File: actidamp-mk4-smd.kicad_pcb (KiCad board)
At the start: 2 copper layers, 119 x 100 mm, 199 parts, among them J101 XLR3, J102 Phono_Ground, J103 PHONO_IN_L, J104 PHONO_IN_R, J105 LINE_OUT_L, J106 LINE_OUT_R, Q201 2SK3320, Q301 2SK3320, Q401 BC846BPN, Q501 BC846BPN, SW201 SW_DIP_x04, SW202 SW_DPDT_x2, SW301 SW_DIP_x04, U101 LM317_3PinPackage, U102 LM337_TO252, U201 NE5532, U202 NE5534, U203 LF411, U204 NE5532, U205 LF411, U301 NE5532, U302 NE5534, U303 LF411, U304 NE5532, U305 LF411

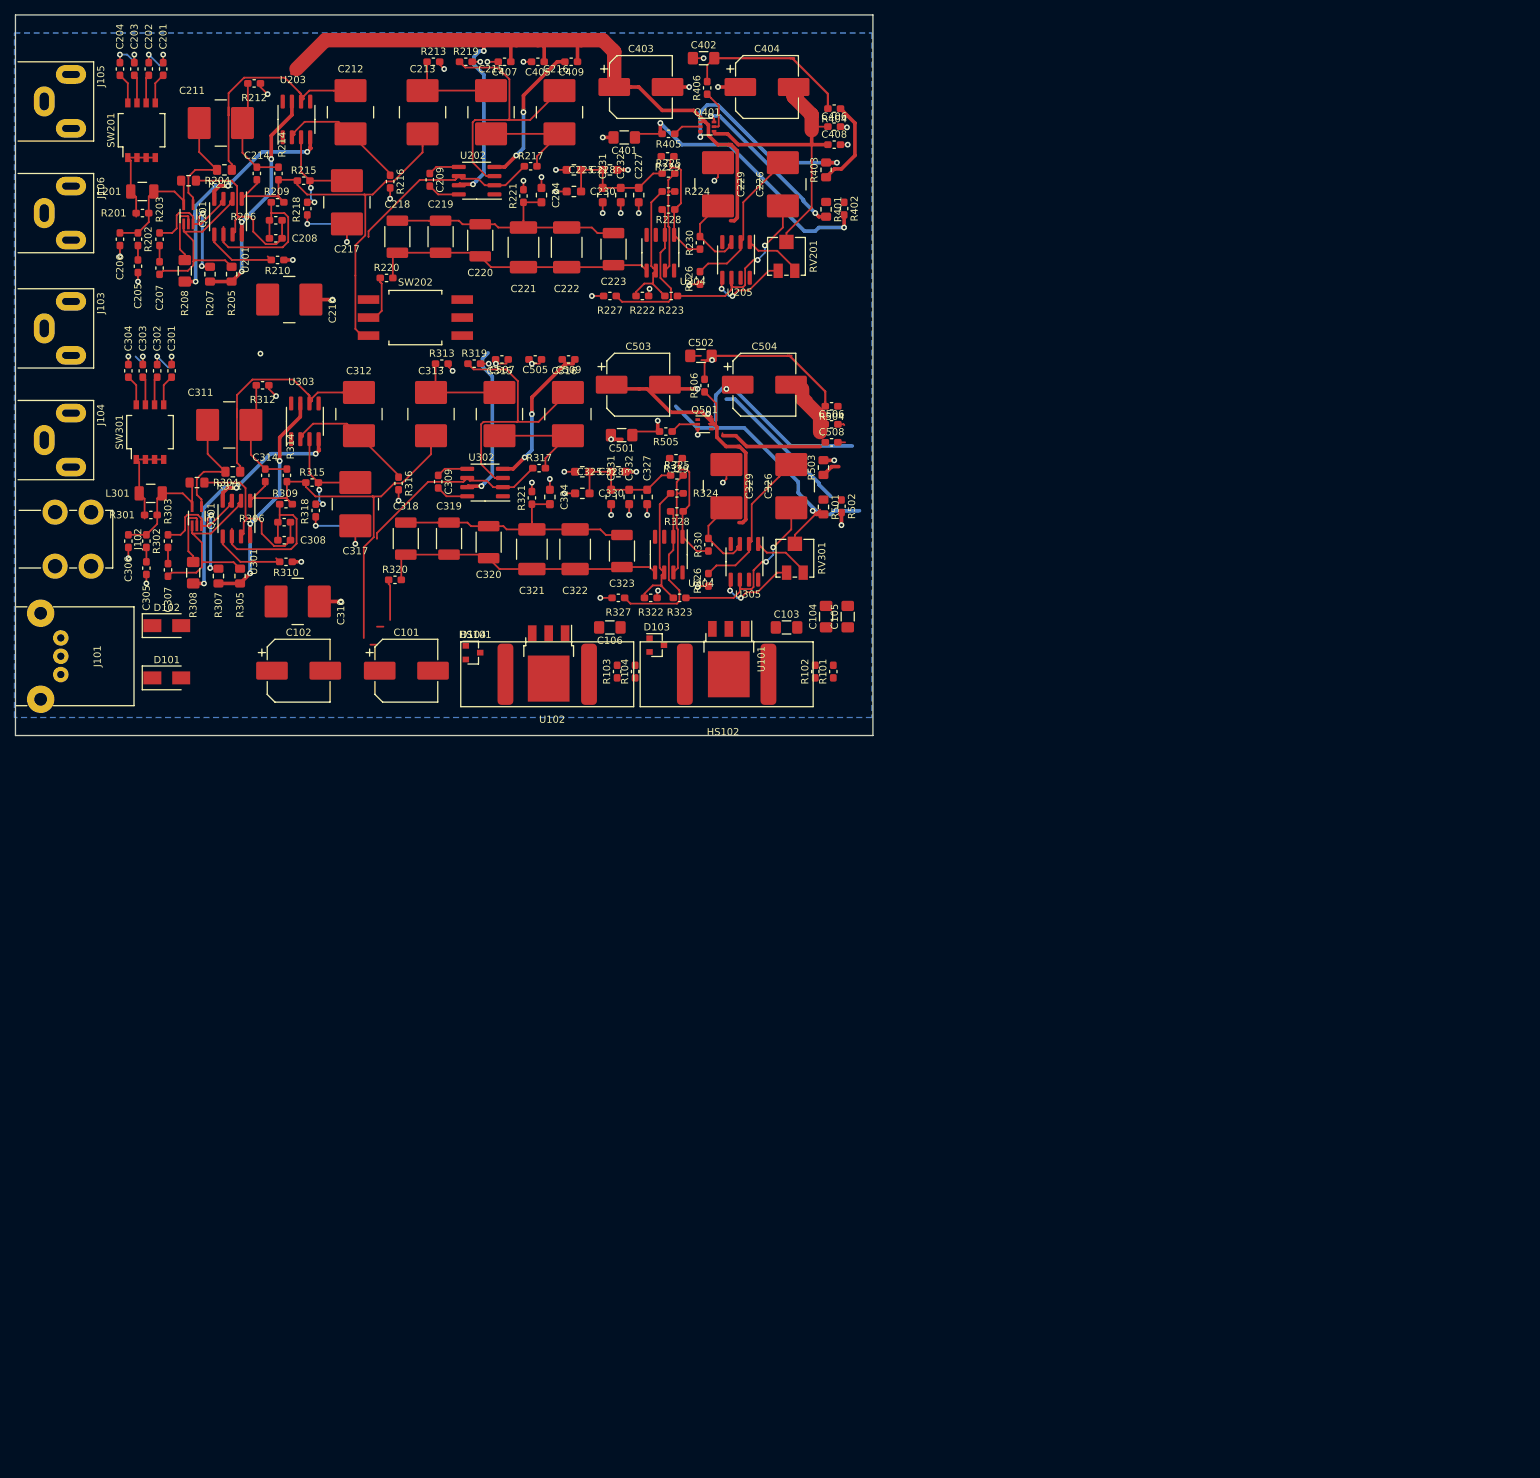
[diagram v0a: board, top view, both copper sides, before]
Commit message: All routed
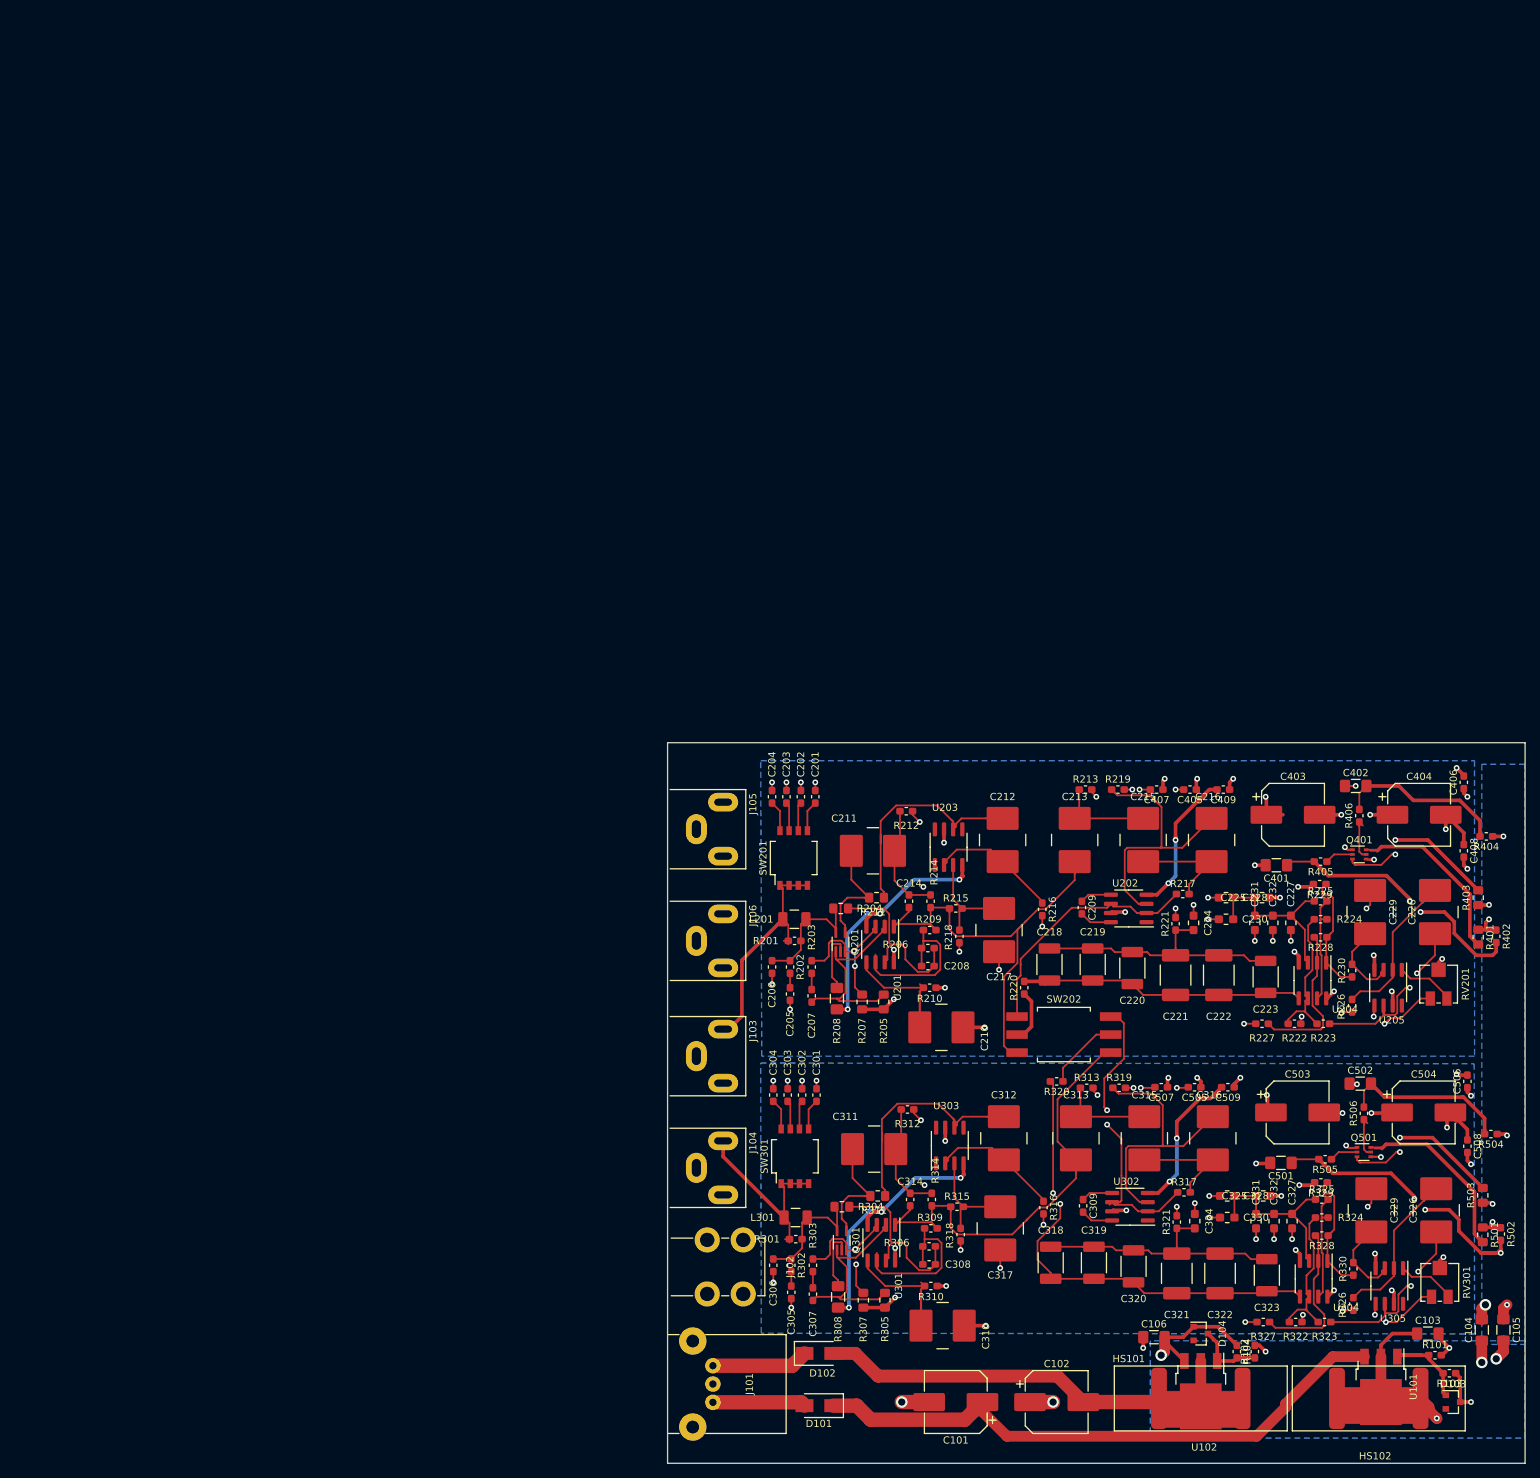
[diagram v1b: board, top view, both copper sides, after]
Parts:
- moved D103 152.5 mm to (199.5, 142.5)
- moved R103 151.1 mm to (199.0, 138.5), turned to 180 degrees
- moved C102 146.2 mm to (144.5, 142.5)
- moved D104 138.3 mm to (164.5, 133.0)
- moved C501 136.3 mm to (175.6, 109.3)
- moved C502 136.3 mm to (186.6, 98.3)
- moved C503 136.3 mm to (177.9, 102.3)
- moved C504 136.3 mm to (195.4, 102.3)
- moved C505 136.3 mm to (163.6, 98.8)
- moved C507 136.3 mm to (159.0, 98.8)
- moved C509 136.3 mm to (168.3, 98.8)
- moved Q501 136.3 mm to (187.1, 107.8)
- moved R501 136.3 mm to (203.6, 119.3)
- moved R502 136.3 mm to (206.1, 119.2)
- moved R503 136.3 mm to (203.6, 113.8)
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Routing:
- net /left_channel/V+: track 152.9 -> 25.1 mm, vias 5 -> 12
- net /right_channel/OUT: track 0.00 -> 104.1 mm, vias 0 -> 1
- net /left_channel/OUT: track 0.00 -> 86.9 mm, vias 0 -> 1
- net Net-(C101-Pad1): track 0.00 -> 83.2 mm
- net Net-(C102-Pad2): track 0.00 -> 67.9 mm
- net /right_channel/V+: track 88.2 -> 25.0 mm, vias 4 -> 12
- net /psu_rails_left/Vreg+: track 0.00 -> 45.6 mm, vias 0 -> 5
- net Net-(C501-Pad1): track 7.34 -> 40.8 mm, vias 2 -> 3
- net /left_channel/V-: track 101.9 -> 73.6 mm, vias 5 -> 11
- net Net-(C318-Pad1): track 39.6 -> 66.8 mm, vias 0 -> 2
- net /left_channel/IN: track 12.5 -> 32.3 mm
- net GND: track 160.0 -> 140.4 mm, vias 66 -> 75
- net /right_channel/IN: track 12.5 -> 28.1 mm
- net Net-(R317-Pad1): track 27.2 -> 42.5 mm, vias 0 -> 2
- net Net-(D103-Pad2): track 0.00 -> 14.1 mm
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- added copper zone on In2.Cu, net /left_channel/V+
- added copper zone on B.Cu, net /left_channel/V-
- added copper zone on In2.Cu, net /psu_rails_left/Vreg+
- added copper zone on B.Cu, net /psu_rails_left/Vreg-
- added copper zone on In2.Cu, net /right_channel/V+
- added copper zone on B.Cu, net /right_channel/V-
- added copper zone on In1.Cu, net GND
- removed copper zone on B.Cu, net GND
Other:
- copper layers 2 -> 4
